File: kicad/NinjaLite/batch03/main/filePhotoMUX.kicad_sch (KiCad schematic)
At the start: 33 parts, among them U19 CD74HC4067M96

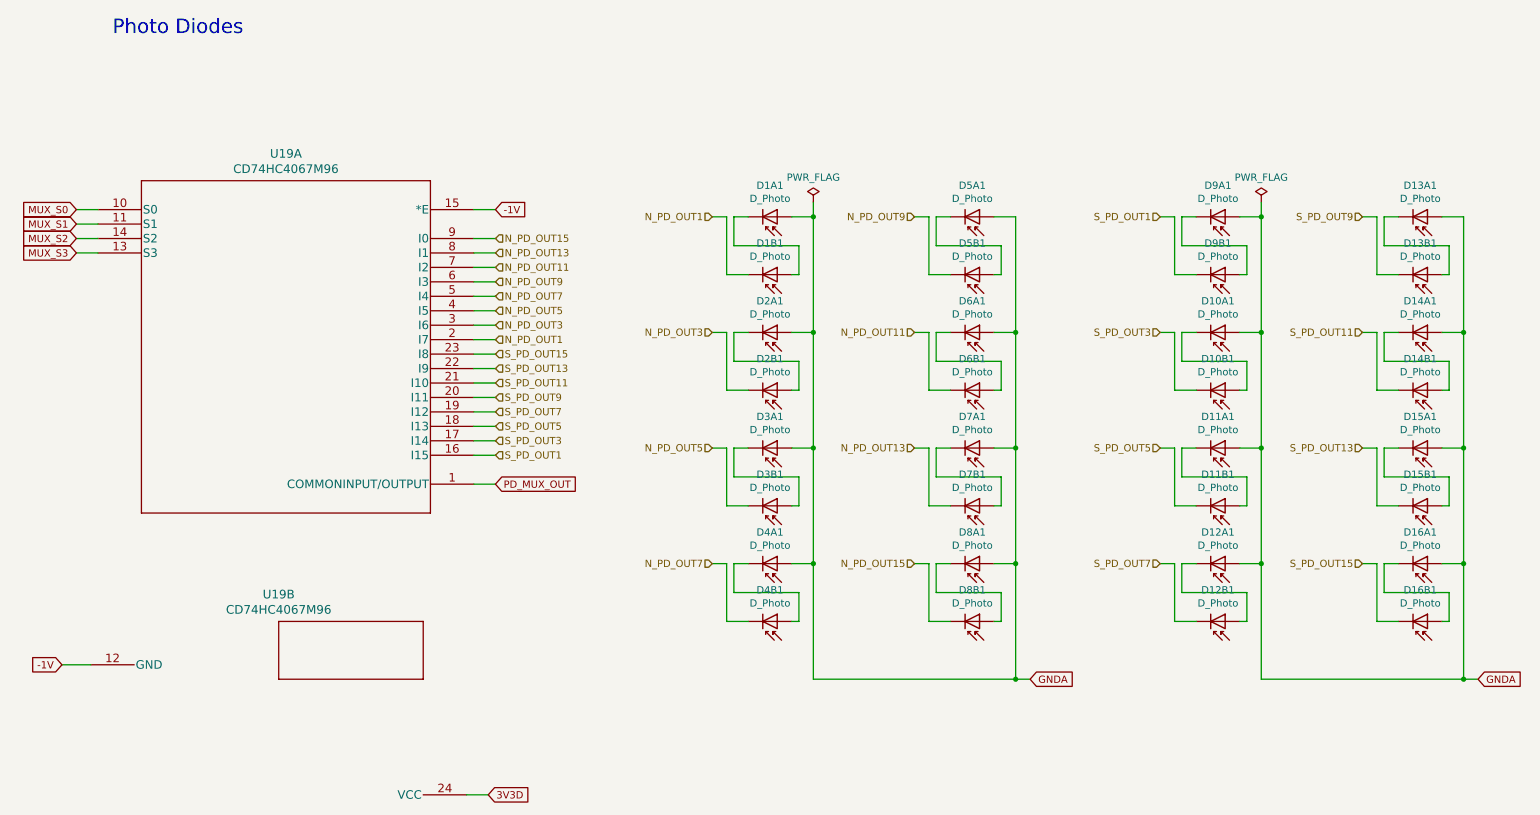
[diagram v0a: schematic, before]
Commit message: just before ripup batch03/main
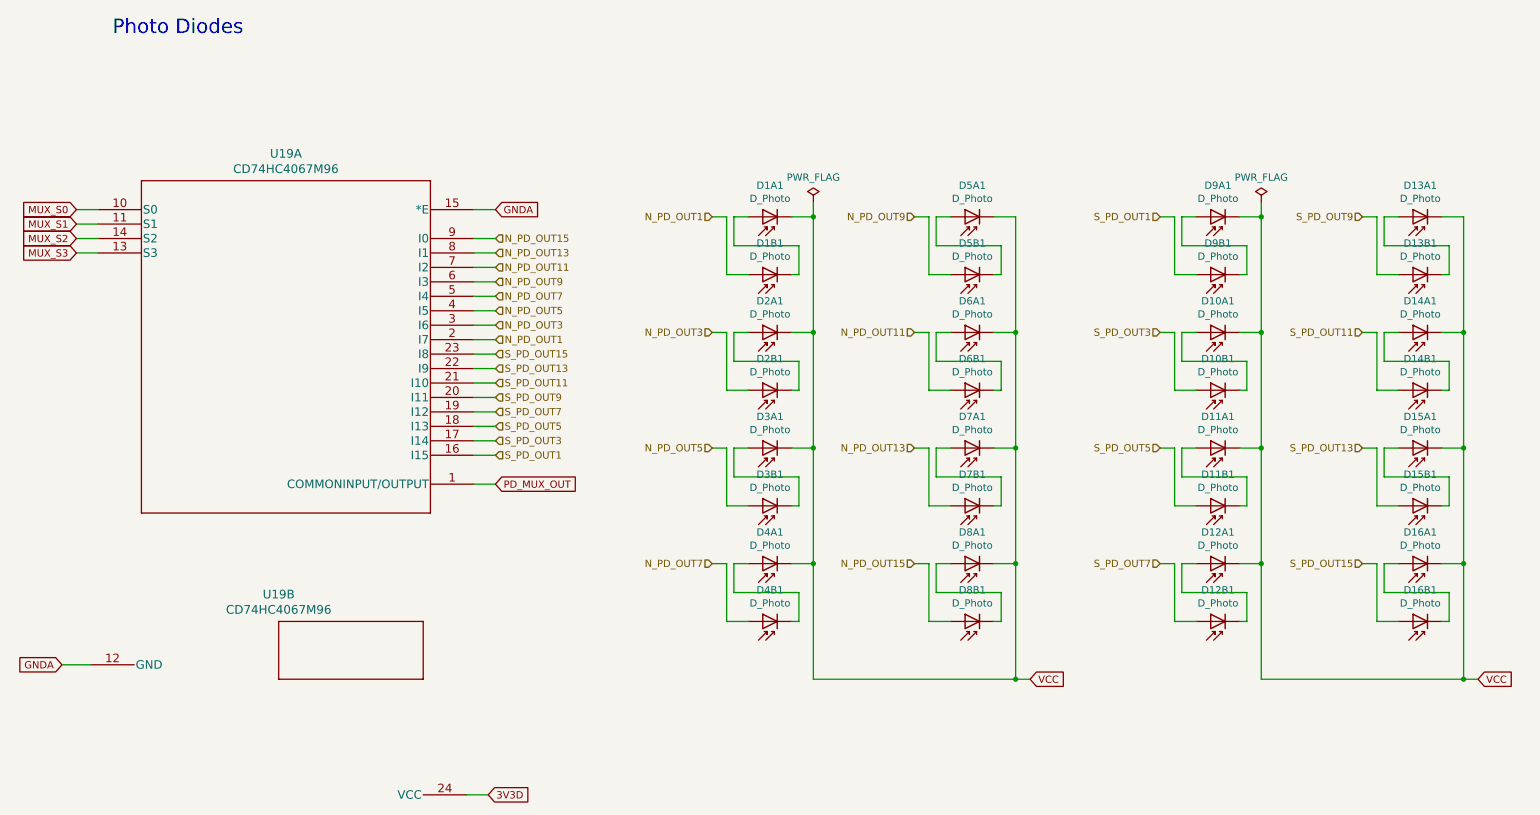
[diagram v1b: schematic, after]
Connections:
- net -1V is gone; now on net GNDA: U19.12 (GND), U19.15 (*E)
- net GNDA: no longer D10A1.2 (A), D11A1.2 (A), D12A1.2 (A), D13A1.2 (A), D14A1.2 (A), D15A1.2 (A), D16A1.2 (A), D1A1.2 (A), D2A1.2 (A), D3A1.2 (A), D4A1.2 (A), D5A1.2 (A), D6A1.2 (A), D7A1.2 (A), D8A1.2 (A), D9A1.2 (A)
- net N_PD_OUT1: now also D1B1.2 (A); no longer D1B1.1 (K)
- net N_PD_OUT11: now also D6B1.2 (A); no longer D6B1.1 (K)
- net N_PD_OUT13: now also D7B1.2 (A); no longer D7B1.1 (K)
- net N_PD_OUT15: now also D8B1.2 (A); no longer D8B1.1 (K)
- net N_PD_OUT3: now also D2B1.2 (A); no longer D2B1.1 (K)
- net N_PD_OUT5: now also D3B1.2 (A); no longer D3B1.1 (K)
- net N_PD_OUT7: now also D4B1.2 (A); no longer D4B1.1 (K)
- net N_PD_OUT9: now also D5B1.2 (A); no longer D5B1.1 (K)
- net S_PD_OUT1: now also D9B1.2 (A); no longer D9B1.1 (K)
- net S_PD_OUT11: now also D14B1.2 (A); no longer D14B1.1 (K)
- net S_PD_OUT13: now also D15B1.2 (A); no longer D15B1.1 (K)
- net S_PD_OUT15: now also D16B1.2 (A); no longer D16B1.1 (K)
- net S_PD_OUT3: now also D10B1.2 (A); no longer D10B1.1 (K)
- net S_PD_OUT5: now also D11B1.2 (A); no longer D11B1.1 (K)
- net S_PD_OUT7: now also D12B1.2 (A); no longer D12B1.1 (K)
- net S_PD_OUT9: now also D13B1.2 (A); no longer D13B1.1 (K)
- net VCC: now reaches D13A1.1 (K)
- net VCC: now also D10A1.1 (K), D11A1.1 (K), D12A1.1 (K), D14A1.1 (K), D15A1.1 (K), D16A1.1 (K), D1A1.1 (K), D2A1.1 (K), D3A1.1 (K), D4A1.1 (K), D5A1.1 (K), D6A1.1 (K), D7A1.1 (K), D8A1.1 (K), D9A1.1 (K); no longer D13B1.2 (A)
- new net: D13A1.2 (A), D13B1.1 (K)
- new net: D5A1.2 (A), D5B1.1 (K)
- new net: D4A1.2 (A), D4B1.1 (K)
- new net: D3A1.2 (A), D3B1.1 (K)
- new net: D9A1.2 (A), D9B1.1 (K)
- new net: D12A1.2 (A), D12B1.1 (K)
- new net: D16A1.2 (A), D16B1.1 (K)
- new net: D15A1.2 (A), D15B1.1 (K)
- new net: D1A1.2 (A), D1B1.1 (K)
- new net: D11A1.2 (A), D11B1.1 (K)
- new net: D2A1.2 (A), D2B1.1 (K)
- new net: D6A1.2 (A), D6B1.1 (K)
- new net: D10A1.2 (A), D10B1.1 (K)
- new net: D14A1.2 (A), D14B1.1 (K)
- new net: D8A1.2 (A), D8B1.1 (K)
- new net: D7A1.2 (A), D7B1.1 (K)
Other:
- moved on the sheet: D10A1, D10B1, D11A1, D11B1, D12A1, D12B1, D13A1, D13B1, D14A1, D14B1, D15A1, D15B1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
